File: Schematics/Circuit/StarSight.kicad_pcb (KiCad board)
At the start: 2 copper layers, 21 parts, among them J10 IR1, J11 IR1, J12 ultSound1, J13 ultSound1, J14 ultSound1, J15 ultSound1, J2 Line1, J3 Line2, J4 Line3, J5 Line4, J6 Line5, J7 IR1, J8 IR1, J9 IR1, P1 CONN_13X2, P2 Power, U1 LM1084IT-5.0/NOPB

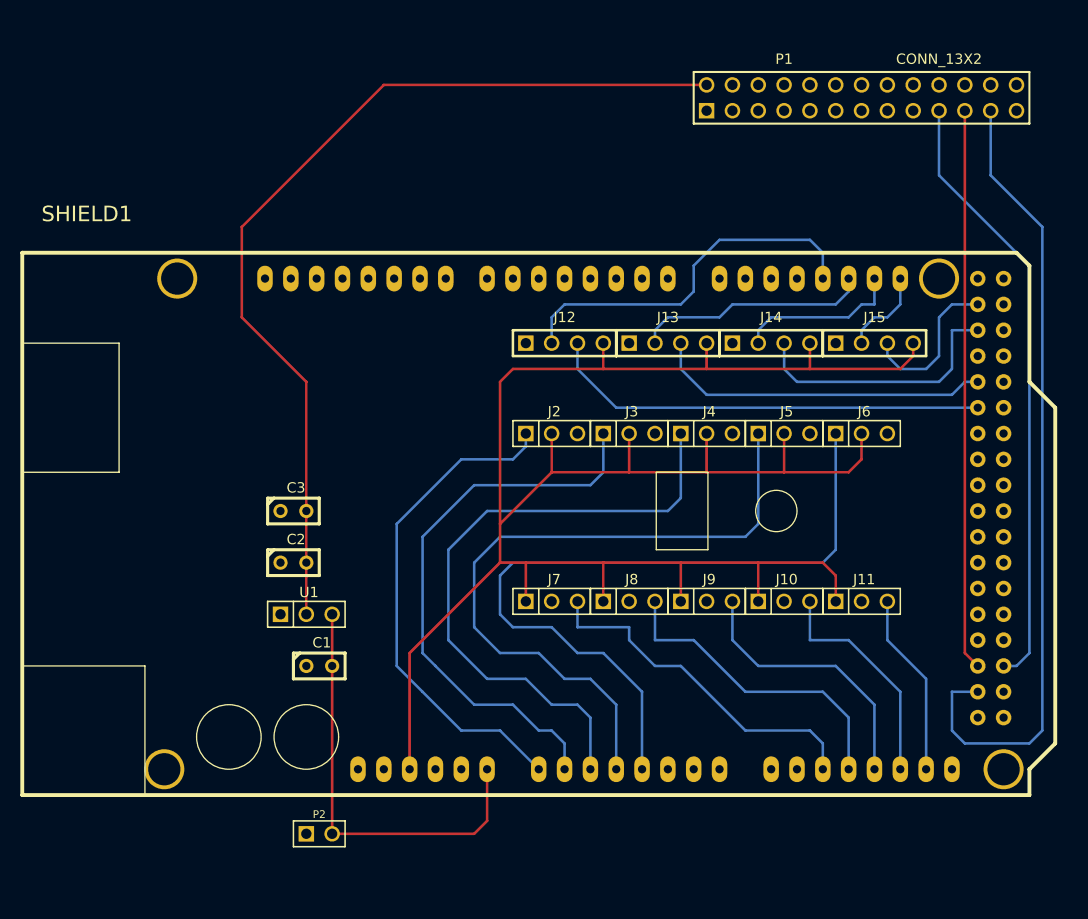
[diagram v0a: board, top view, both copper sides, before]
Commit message: Fix pcb
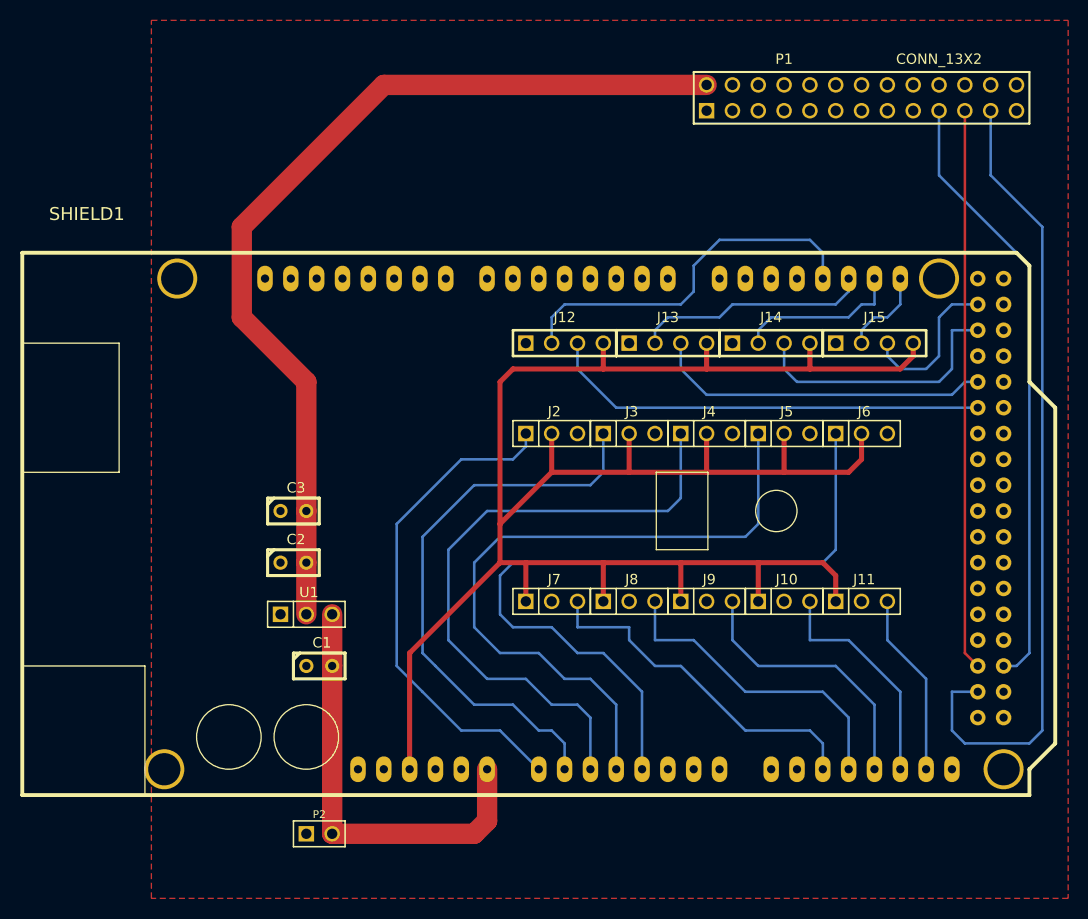
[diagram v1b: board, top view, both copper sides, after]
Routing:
- added copper zone on F.Cu, net GND
